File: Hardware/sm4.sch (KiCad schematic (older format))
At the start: 94 parts, among them J1 Motor1, J2 Termination, J3 CAN bus, J4 Motor2, J5 I2C, J6 Power, J7 USB_C_Receptacle_USB2.0, Q1 NDT2955, SW1 RST_SW, SW2 BOOT_SW, U1 STM32F412RETx, U2 TMC2100-TA, U3 MCP2562-E-SN, U4 TMC2100-TA, U5 LM2594HVM-5.0, U6 MCP1700-3302E_SOT23, U7 USBLC6-2SC6, Y1 25 MHz

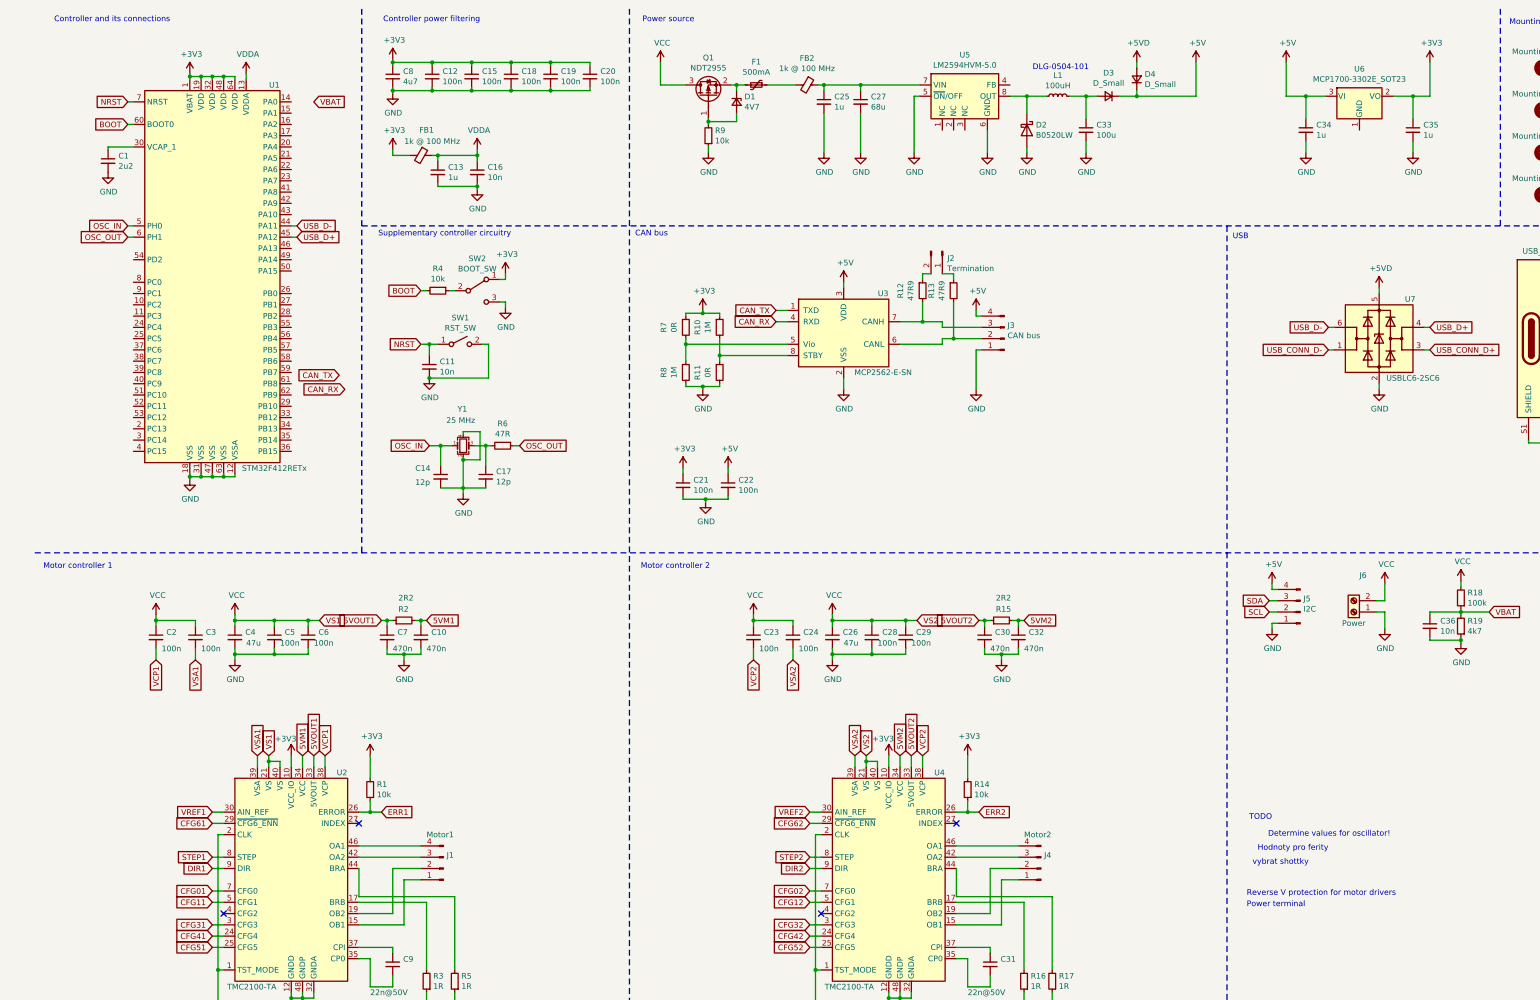
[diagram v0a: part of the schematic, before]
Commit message: Finish first version of the PCB, which is trash and shall perish.
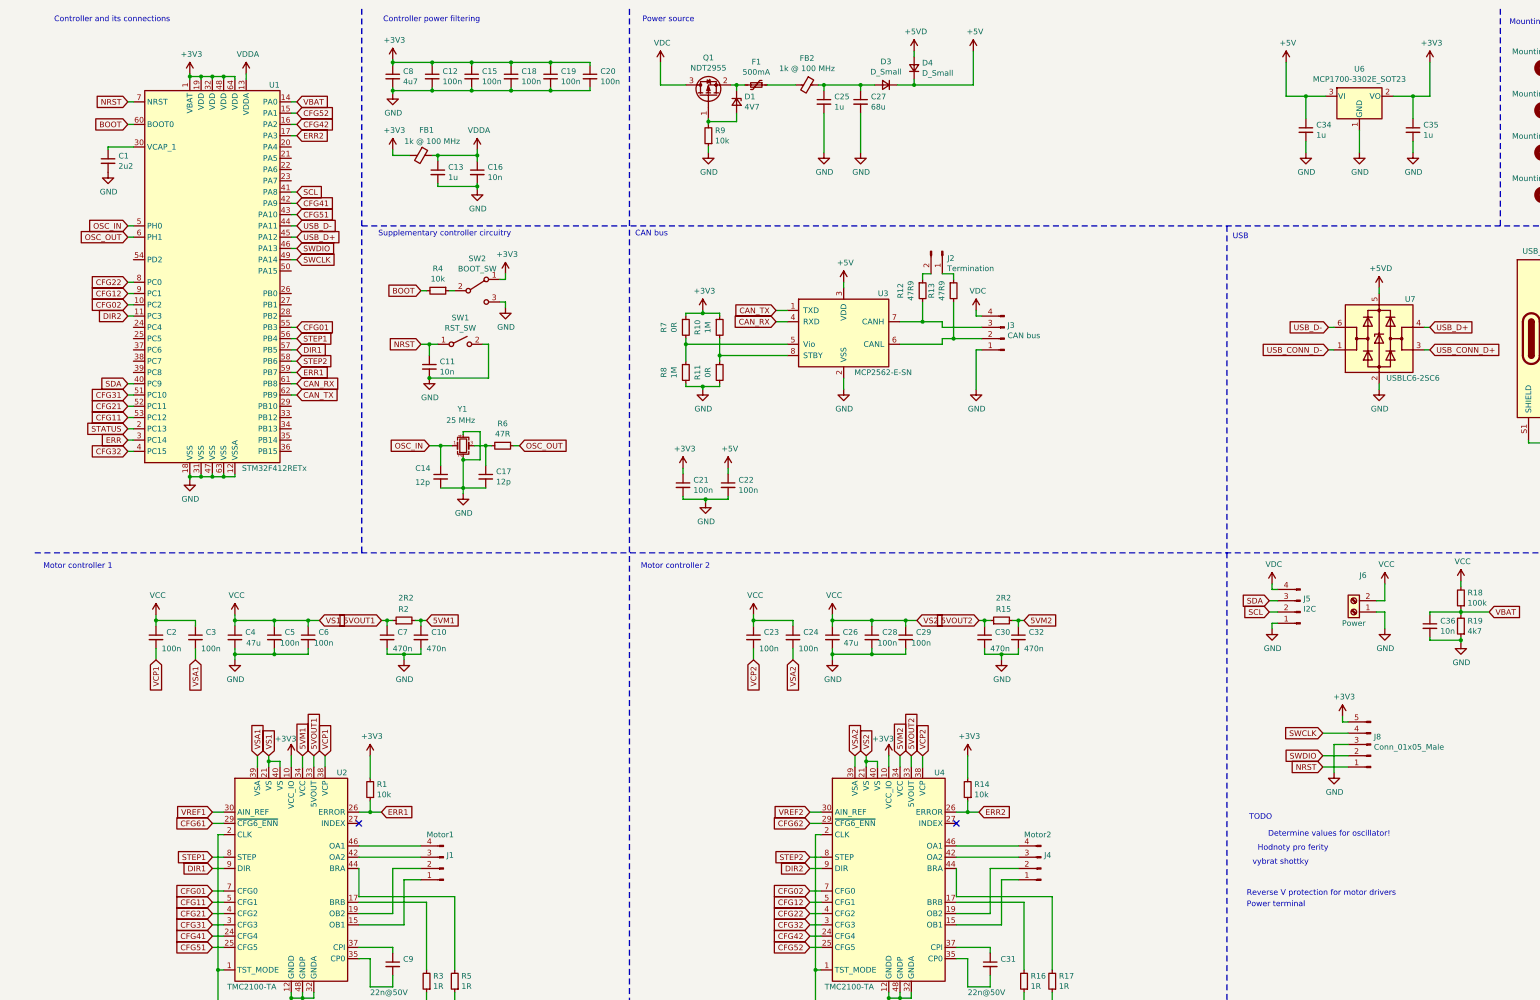
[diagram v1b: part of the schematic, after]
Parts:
- removed C33: 100u, Capacitor_SMD:C_Elec_6.3x5.8, symbol Device:C_Small
- removed D2: B0520LW, Diode_SMD:D_SOD-123, symbol Diode:1N5817
- removed L1: 100uH, Inductor_SMD:L_Wuerth_HCI-1050, symbol Device:L_Small
- removed U5: LM2594HVM-5.0, Package_SO:SOIC-8_3.9x4.9mm_P1.27mm, symbol Regulator_Switching:LM2594HVM-5.0
- added J8: Conn_01x05_Male, Connector_Molex:Molex_SPOX_5267-05A_1x05_P2.50mm_Vertical, symbol Connector:Conn_01x05_Male
- C10, C30, C32, C7: footprint Capacitor_SMD:C_0805_2012Metric_Pad1.18x1.45mm_HandSolder -> Capacitor_SMD:C_0603_1608Metric_Pad1.08x0.95mm_HandSolder
- F1: footprint Fuse:Fuse_2920_7451Metric_Pad2.10x5.45mm_HandSolder -> Fuse:Fuse_1206_3216Metric_Pad1.42x1.75mm_HandSolder
- SW1: footprint Button_Switch_SMD:SW_Push_1P1T_NO_6x6mm_H9.5mm -> Connector_PinHeader_2.54mm:PinHeader_1x02_P2.54mm_Vertical
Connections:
- net +3V3: now also J8.5 (Pin_5)
- net +5V: no longer J3.4 (Pin_4), J5.4 (Pin_4)
- net CAN_RX: now also U1.61 (PB8)
- net CAN_TX: now also U1.62 (PB9)
- net CFG01: now also U1.55 (PB3)
- net CFG02: now also U1.10 (PC2)
- net CFG11: now also U1.53 (PC12)
- net CFG12: now also U1.9 (PC1)
- net CFG31: now also U1.51 (PC10)
- net CFG32: now also U1.4 (PC15)
- net CFG41: now also U1.42 (PA9)
- net CFG42: now also U1.16 (PA2)
- net CFG51: now also U1.43 (PA10)
- net CFG52: now also U1.15 (PA1)
- net DIR1: now also U1.57 (PB5)
- net DIR2: now also U1.11 (PC3)
- net ERR: now also U1.3 (PC14)
- net ERR1: now also U1.59 (PB7)
- net ERR2: now also U1.17 (PA3)
- net GND: now also U6.1 (GND), J8.3 (Pin_3)
- net NRST: now also J8.1 (Pin_1)
- net SCL: now also U1.41 (PA8)
- net SDA: now also U1.40 (PC9)
- net STATUS: now also U1.2 (PC13)
- net STEP1: now also U1.56 (PB4)
- net STEP2: now also U1.58 (PB6)
- net VBAT: now also U1.14 (PA0)
- net VCC: no longer Q1.3 (D)
- net SWDIO: now reaches U1.46 (PA13)
- net SWDIO: now also J8.2 (Pin_2)
- net SWCLK: now reaches U1.49 (PA14)
- net SWCLK: now also J8.4 (Pin_4)
- net CFG21: now reaches U1.52 (PC11)
- net CFG21: now also U2.4 (CFG2)
- net CFG22: now reaches U1.8 (PC0)
- net CFG22: now also U4.4 (CFG2)
- net at C25.1, C27.1, FB2.1: now also D3.2 (A)
- new net VDC: J3.4 (Pin_4), J5.4 (Pin_4), Q1.3 (D)
- no-connect marks 6 -> 4
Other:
- note removed: "DLG-0504-101"
- moved on the sheet: D3, D4
